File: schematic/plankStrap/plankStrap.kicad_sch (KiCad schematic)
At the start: 3 parts, among them U1 Xplained_328p, U2 Gyro_Absolute_BNO055, U3 LCD_2.4in_ILI9341

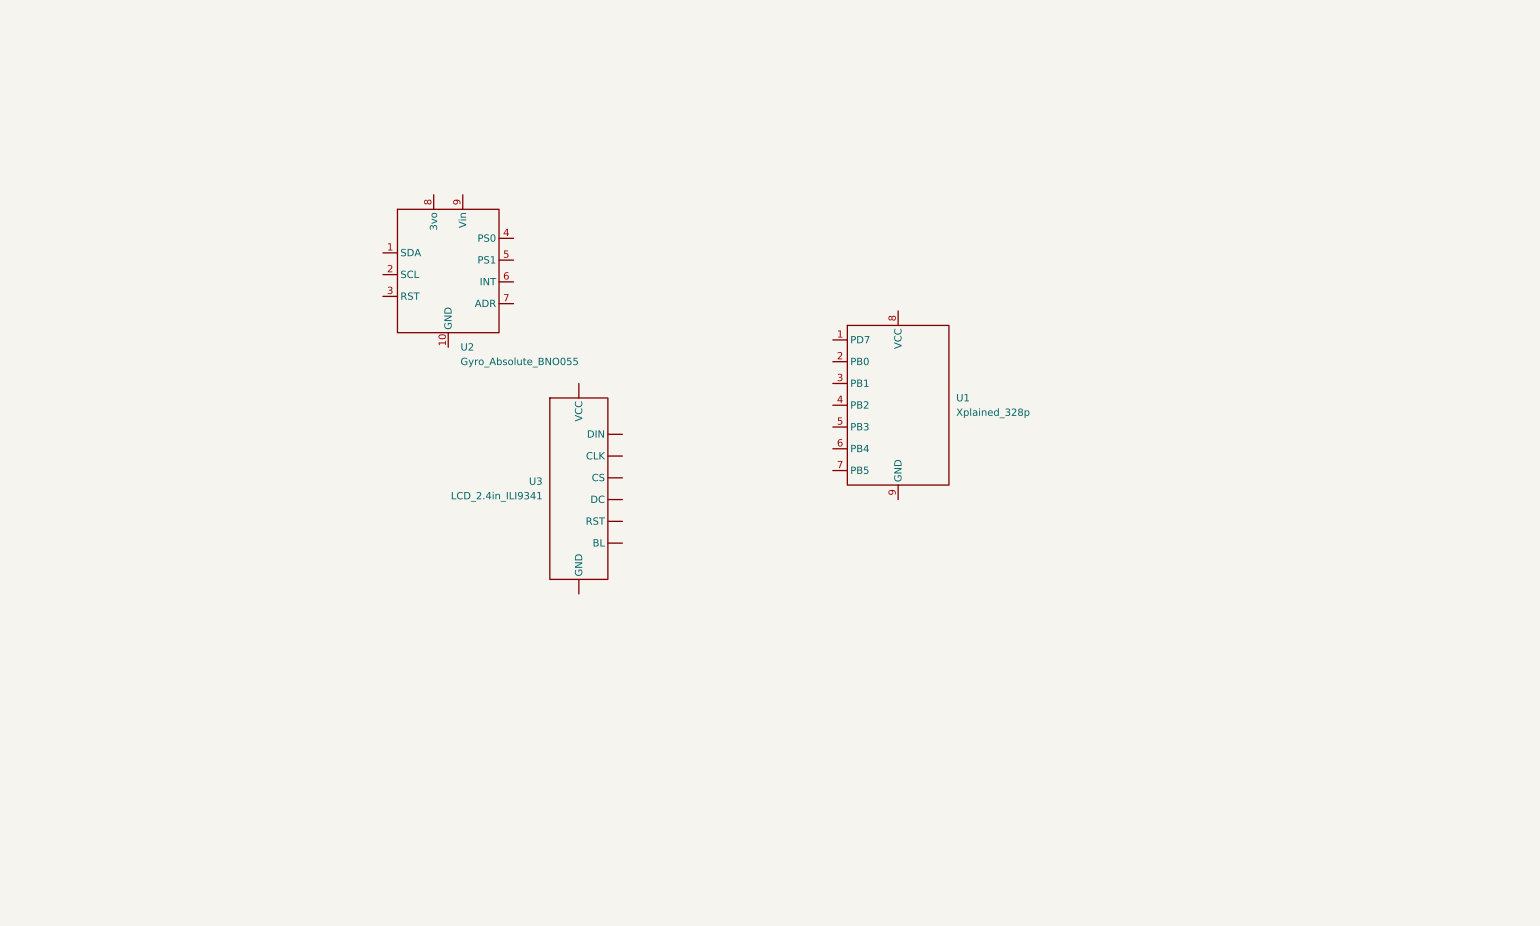
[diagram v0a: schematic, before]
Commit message: schematic v1
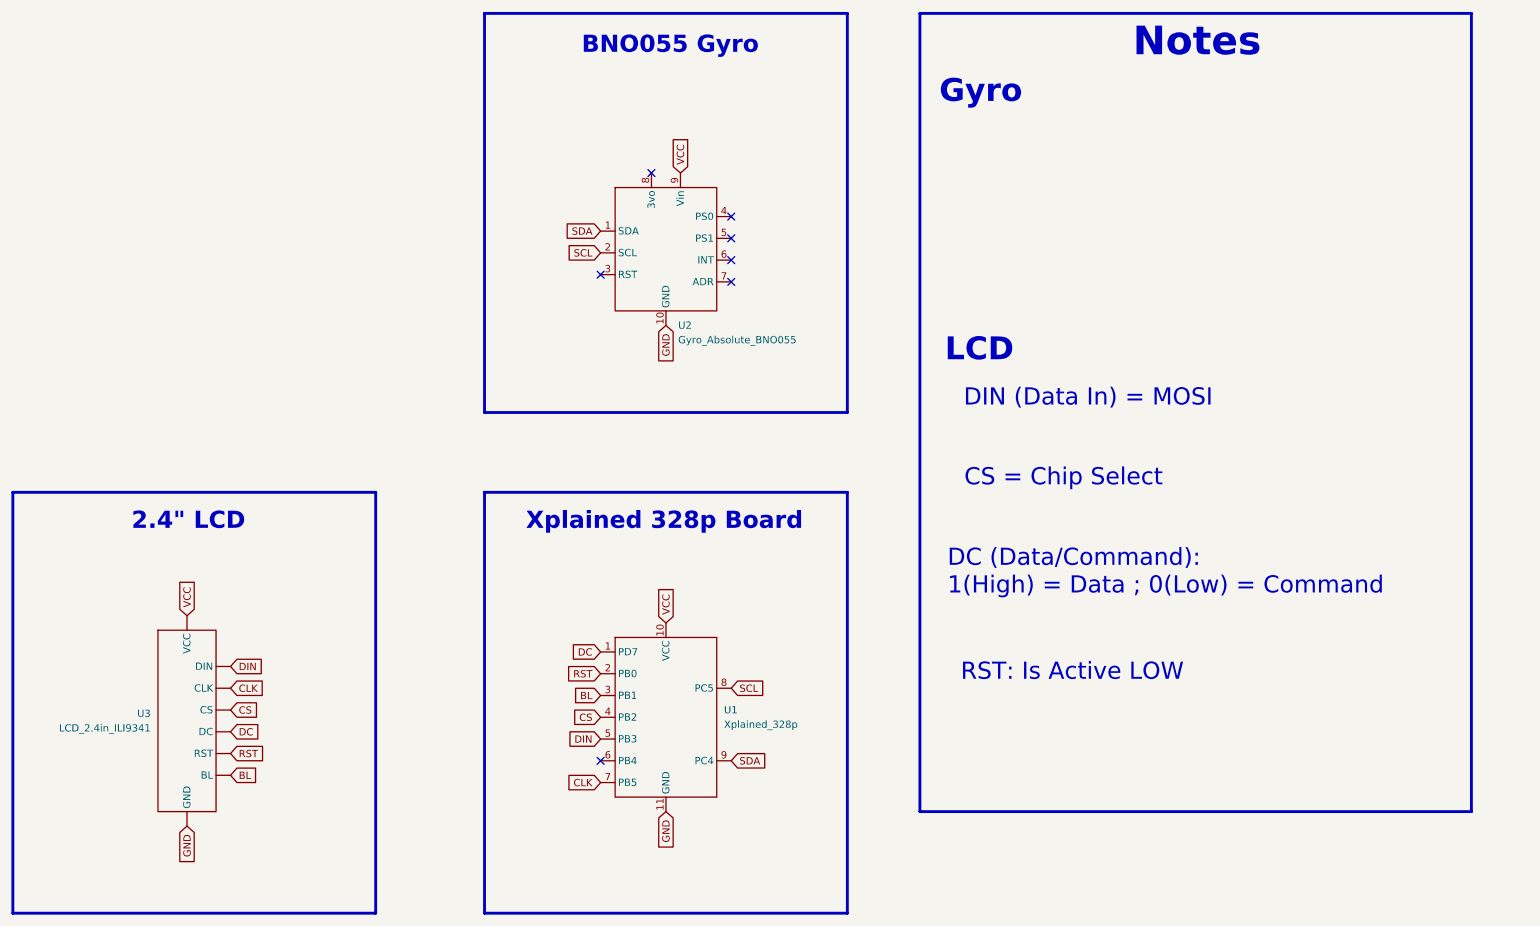
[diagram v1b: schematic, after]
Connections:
- net DC: now reaches U1.1 (PD7)
- net DC: now also U3. (BL)
- net RST: now reaches U1.2 (PB0)
- net RST: now also U3. (BL)
- net BL: now reaches U1.3 (PB1)
- net BL: now also U3. (BL)
- net CS: now reaches U1.4 (PB2)
- net CS: now also U3. (BL)
- net DIN: now reaches U1.5 (PB3)
- net DIN: now also U3. (BL)
- net CLK: now reaches U1.7 (PB5)
- net CLK: now also U3. (BL)
- net SCL: now reaches U1.8 (PC5)
- net SCL: now also U2.2 (SCL)
- net SDA: now reaches U1.9 (PC4)
- net SDA: now also U2.1 (SDA)
- net GND: now reaches U2.10 (GND)
- net GND: now also U1.11 (GND), U3. (BL)
- net VCC: now reaches U2.9 (Vin)
- net VCC: now also U1.10 (VCC), U3. (BL)
- no-connect marks 0 -> 7
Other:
- note added: "2.4" LCD"
- note added: "BNO055 Gyro"
- note added: "CS = Chip Select"
- note added: "DC (Data/Command): 1(High) = Data ; 0(Low) = Command"
- note added: "DIN (Data In) = MOSI"
- note added: "Gyro"
- note added: "LCD"
- note added: "Notes"
- note added: "RST: Is Active LOW"
- note added: "Xplained 328p Board"
- moved on the sheet: U2, U3
